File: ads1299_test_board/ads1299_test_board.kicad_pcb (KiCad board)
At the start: 2 copper layers, 67.7 x 57.4 mm, 63 parts, among them CN1 W2A45C103MAT2A, CN2 W2A45C103MAT2A, IC1 TPS61023DRLR, IC2 TPS7A2050PDBVR, J1 Conn_01x02, J3 Conn_02x05_Top_Bottom, P1 USB_C_Plug_USB2.0, Q1 AO3407A, SW1 EG1218, SW2 PTS810SJM250SMTR LFS, U1 ADS1299, U2 MCP73832-2-OT, U3 ESP32-S3-WROOM-1, U4 OPA376xxD, U6 AP2112K-3.3, U7 TPD4E05U06DQA

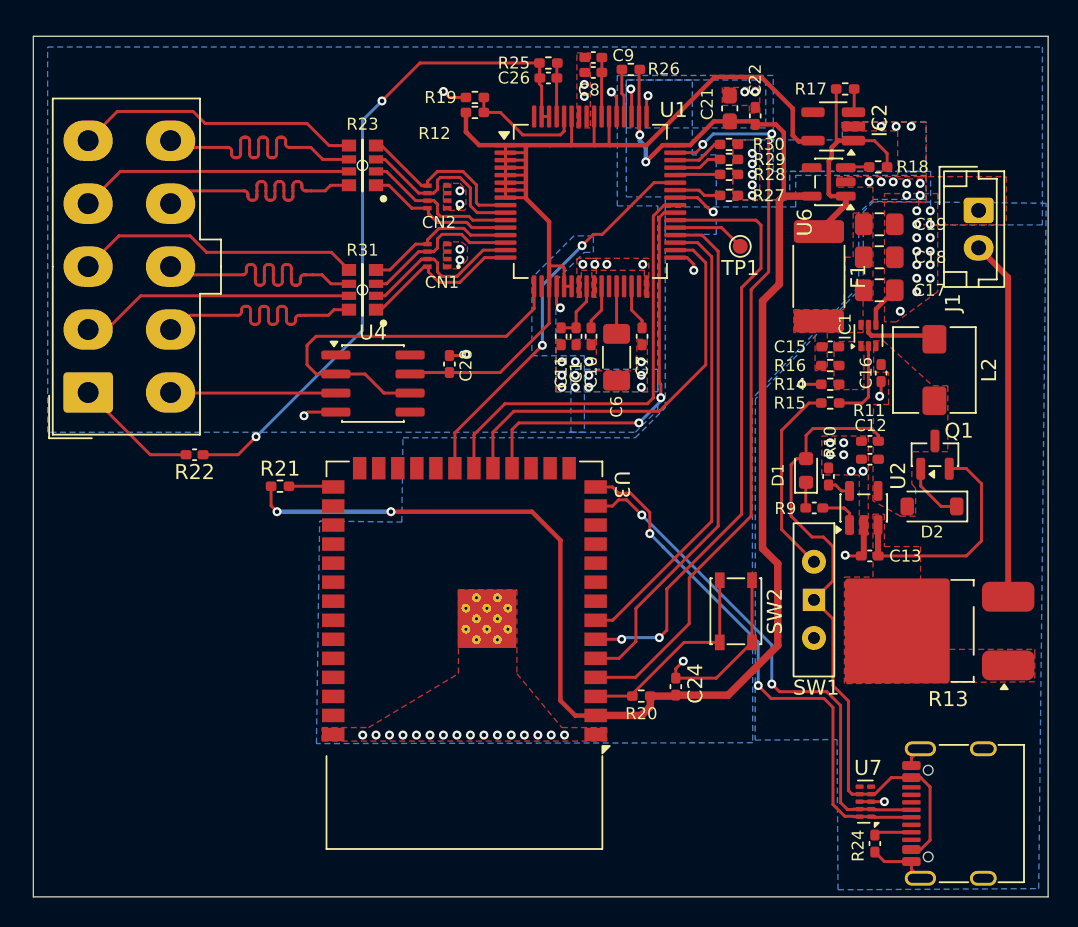
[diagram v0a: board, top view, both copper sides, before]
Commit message: 8 channel
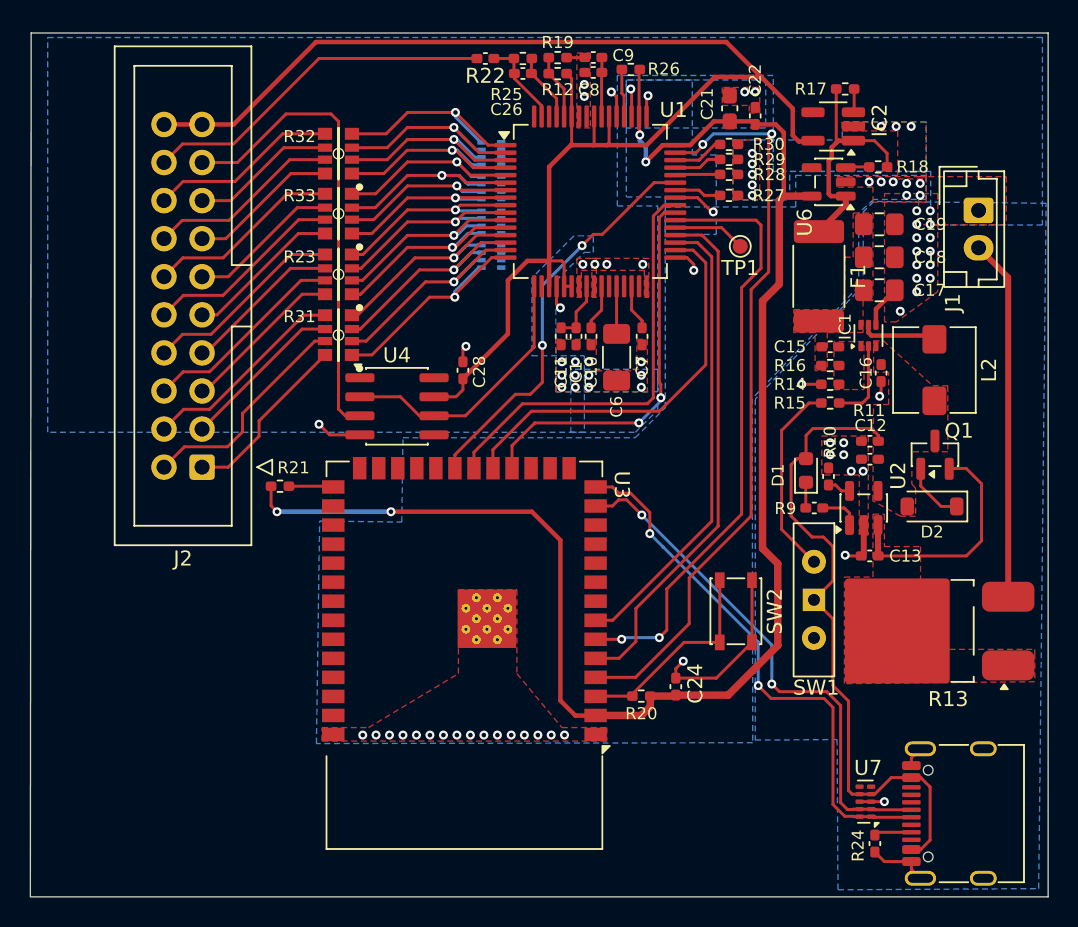
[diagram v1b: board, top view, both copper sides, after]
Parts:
- removed J3: Conn_02x05_Top_Bottom, Connector_Molex:Molex_Mini-Fit_Jr_5566-10A_2x05_P4.20mm_Vertical
- added CN3: W2A45C103MAT2A, W2A45C103MAT2A:W2A45C103MAT2A, B.Cu at (136.6, 81.2)
- added CN4: W2A45C103MAT2A, W2A45C103MAT2A:W2A45C103MAT2A, B.Cu at (136.6, 78.9)
- added J2: Conn_02x10_Counter_Clockwise, Connector_IDC:IDC-Header_2x10_P2.54mm_Vertical, F.Cu at (117.3, 99.9)
- added R32: CAY16-2201F4LF, CAY16-2201F4LF:RESCAX80P160X320X60-8N, F.Cu at (126.4, 79.0)
- added R33: CAY16-2201F4LF, CAY16-2201F4LF:RESCAX80P160X320X60-8N, F.Cu at (126.4, 83.0)
- CN1, CN2: moved to B.Cu
- moved R22 32.8 mm to (136.2, 72.6)
- moved R23 7.44 mm to (126.4, 87.0)
- moved R19 6.13 mm to (141.0, 72.5), turned to 0 degrees
- moved R12 6.10 mm to (141.0, 73.6), turned to 180 degrees
- moved CN2 3.97 mm to (136.6, 83.5), turned to -90 degrees
- moved CN1 3.60 mm to (136.6, 85.8), turned to -90 degrees
- moved R31 3.42 mm to (126.4, 91.0)
- moved U4 2.21 mm to (130.3, 95.8)
- moved C26 1.73 mm to (138.7, 73.6)
- moved R25 1.73 mm to (138.7, 72.6)
- moved C28 0.99 mm to (134.7, 93.4)
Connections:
- CN1 pad 5: /ads1299_AFE_/2N -> /ads1299_AFE_/1P
- CN1 pad 6: /ads1299_AFE_/2P -> /ads1299_AFE_/1N
- CN1 pad 7: /ads1299_AFE_/1N -> /ads1299_AFE_/2P
- CN1 pad 8: /ads1299_AFE_/1P -> /ads1299_AFE_/2N
- CN2 pad 5: /ads1299_AFE_/4N -> /ads1299_AFE_/3P
- CN2 pad 6: /ads1299_AFE_/4P -> /ads1299_AFE_/3N
- CN2 pad 7: /ads1299_AFE_/3N -> /ads1299_AFE_/4P
- CN2 pad 8: /ads1299_AFE_/3P -> /ads1299_AFE_/4N
- U1 pad 1: /ads1299_AFE_/AVDD -> /ads1299_AFE_/8N
- U1 pad 2: /ads1299_AFE_/AVDD -> /ads1299_AFE_/8P
- U1 pad 3: /ads1299_AFE_/AVDD -> /ads1299_AFE_/7N
- U1 pad 4: /ads1299_AFE_/AVDD -> /ads1299_AFE_/7P
- U1 pad 5: /ads1299_AFE_/AVDD -> /ads1299_AFE_/6N
- U1 pad 6: /ads1299_AFE_/AVDD -> /ads1299_AFE_/6P
- U1 pad 7: /ads1299_AFE_/AVDD -> /ads1299_AFE_/5N
- U1 pad 8: /ads1299_AFE_/AVDD -> /ads1299_AFE_/5P
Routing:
- net /ads1299_AFE_/Bias_out: track 46.6 -> 5.97 mm, vias 2 -> 0
- net /ads1299_AFE_/AVDD: track 74.5 -> 99.9 mm
- net /ads1299_AFE_/Ref_electrode: track 11.0 -> 31.4 mm
- net /ads1299_AFE_/Bias_electrode: track 8.25 -> 23.7 mm
- net /ads1299_AFE_/8N: track 0.00 -> 14.5 mm, vias 0 -> 1
- net /ads1299_AFE_/6P: track 0.00 -> 14.3 mm, vias 0 -> 1
- net /ads1299_AFE_/8P: track 0.00 -> 14.0 mm, vias 0 -> 1
- net /ads1299_AFE_/7P: track 0.00 -> 13.7 mm, vias 0 -> 1
- net /ads1299_AFE_/7N: track 0.00 -> 13.7 mm, vias 0 -> 1
- net /ads1299_AFE_/6N: track 0.00 -> 13.5 mm, vias 0 -> 1
- net /ads1299_AFE_/IN5N: track 0.00 -> 13.4 mm
- net /ads1299_AFE_/5N: track 0.00 -> 13.1 mm, vias 0 -> 1
- net /ads1299_AFE_/IN6N: track 0.00 -> 13.0 mm
- net /ads1299_AFE_/5P: track 0.00 -> 13.0 mm, vias 0 -> 1
- net /ads1299_AFE_/IN7N: track 0.00 -> 12.9 mm
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- removed copper zone on B.Cu, net (none)
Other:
- board size 67.7 x 57.4 mm -> 67.9 x 57.6 mm
